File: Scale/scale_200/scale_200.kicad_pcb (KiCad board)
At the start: 2 copper layers, 205 x 20 mm, 39 parts, among them J1 Conn_ARM_JTAG_SWD_10, J2 Conn_01x06_Socket, J3 12V PSU, J4 Conn_01x03_Socket, J5 Conn_01x06_Socket, U1 STM32F103C8Tx, U2 W25Q32JVSS, U3 MC33063AD

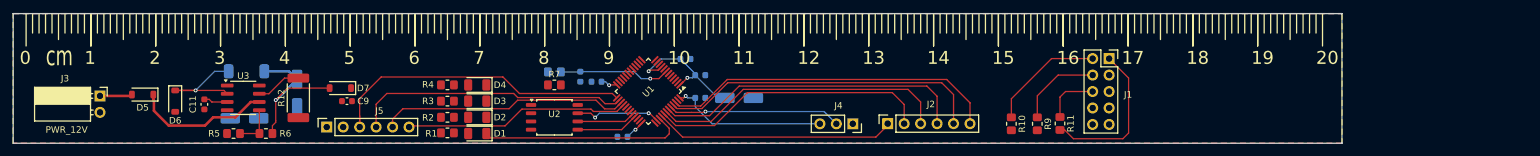
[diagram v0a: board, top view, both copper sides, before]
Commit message: scale done. Just GERBER left
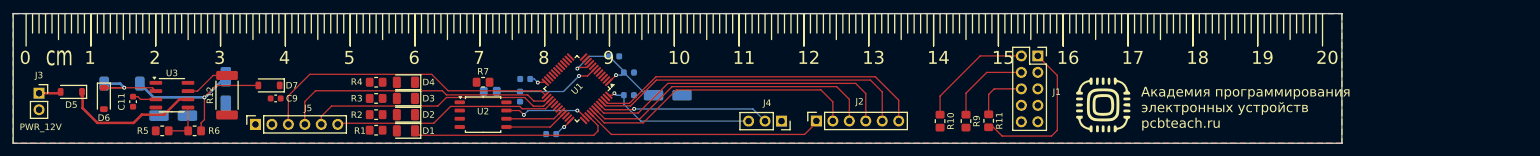
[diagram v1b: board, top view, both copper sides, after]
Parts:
- added G***: LOGO, LOGO, F.Cu at (236.2, 124.0)
- added G***: LOGO, LOGO, B.Cu at (264.4, 123.4)
- J3: footprint Connector_PinSocket_2.54mm:PinSocket_1x02_P2.54mm_Horizontal -> Connector_PinSocket_2.54mm:PinSocket_1x02_P2.54mm_Vertical
- moved L1 19.3 mm to (84.8, 120.8)
- moved C1 11.0 mm to (163.0, 122.6)
- moved C11 11.0 mm to (86.5, 123.6)
- moved C2 11.0 mm to (151.0, 128.6)
- moved C3 11.0 mm to (147.0, 120.1)
- moved C4 11.0 mm to (163.0, 119.1)
- moved C5 11.0 mm to (160.7, 116.6)
- moved C6 11.0 mm to (169.0, 122.6)
- moved C7 11.0 mm to (92.7, 125.7)
- moved C8 11.0 mm to (100.8, 121.9)
- moved C9 11.0 mm to (108.5, 123.1)
- moved D1 11.0 mm to (128.6, 128.1)
- moved D2 11.0 mm to (128.6, 125.6)
- moved D3 11.0 mm to (128.6, 123.1)
- moved D4 11.0 mm to (128.6, 120.6)
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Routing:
- net Net-(D7-A): track 24.8 -> 30.0 mm
- net Net-(D6-K): track 17.7 -> 14.8 mm
- net Net-(D5-A): track 5.01 -> 3.41 mm
- net /NRST: track 17.2 -> 16.7 mm
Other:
- board text added: "Академия программирования электронных устройств pcbteach.ru"

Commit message: box bottom done. gerber generated OK
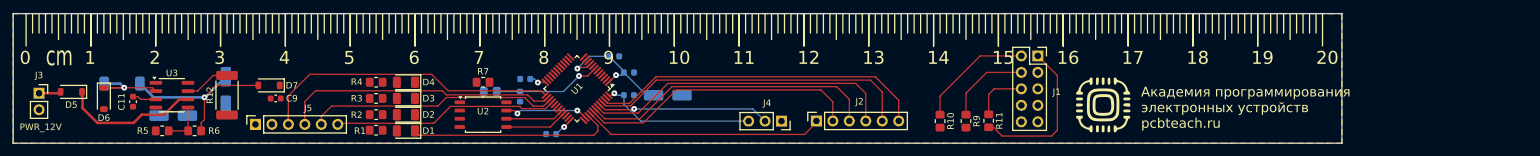
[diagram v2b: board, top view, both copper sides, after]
